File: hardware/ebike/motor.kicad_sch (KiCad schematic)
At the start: 48 parts, among them J2 Screw_Terminal_01x03, Q2 CSD19532KTT, Q3 CSD19532KTT, Q4 CSD19532KTT, Q5 CSD19532KTT, Q6 CSD19532KTT, Q7 CSD19532KTT

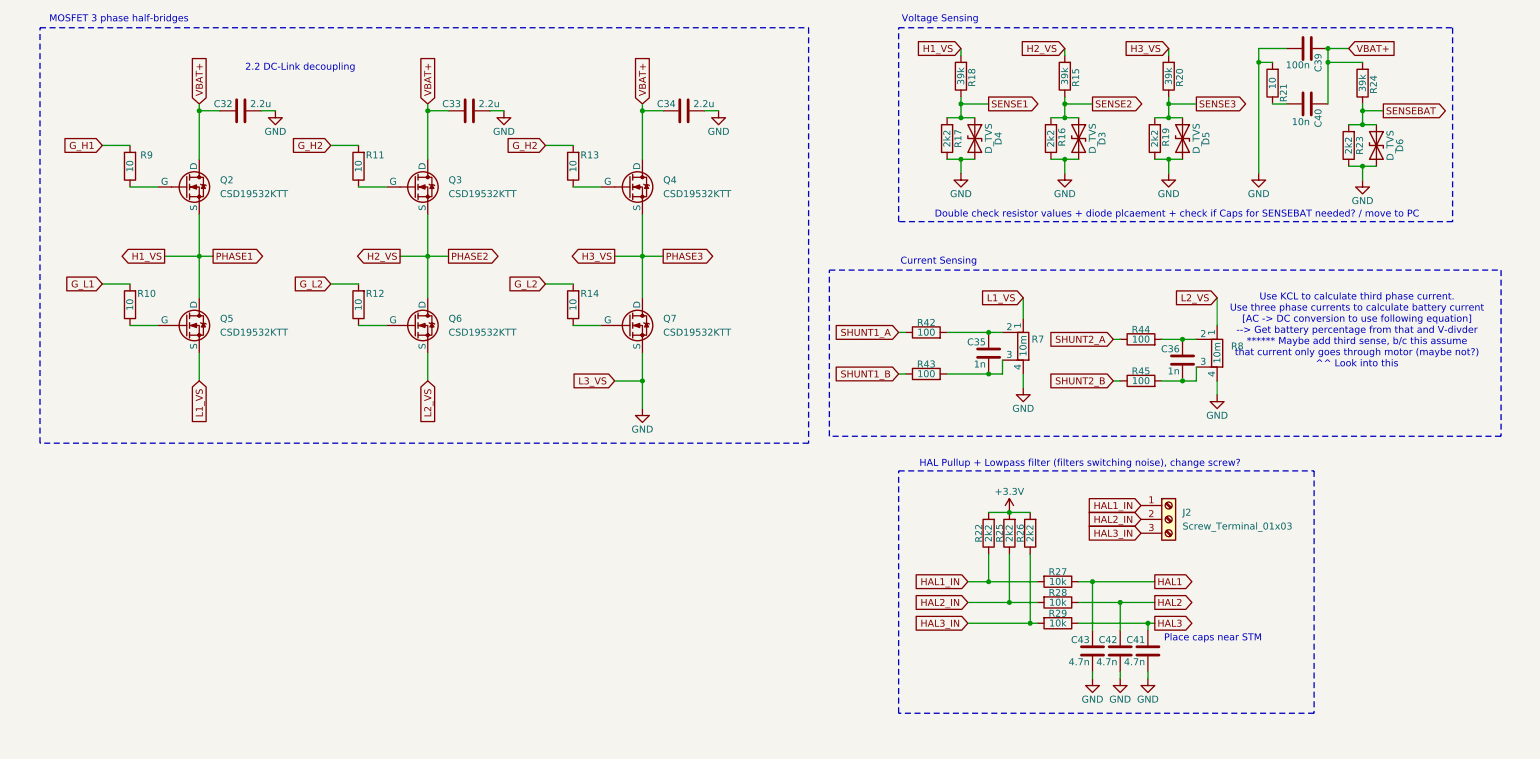
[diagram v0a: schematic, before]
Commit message: finished annoation for schematic
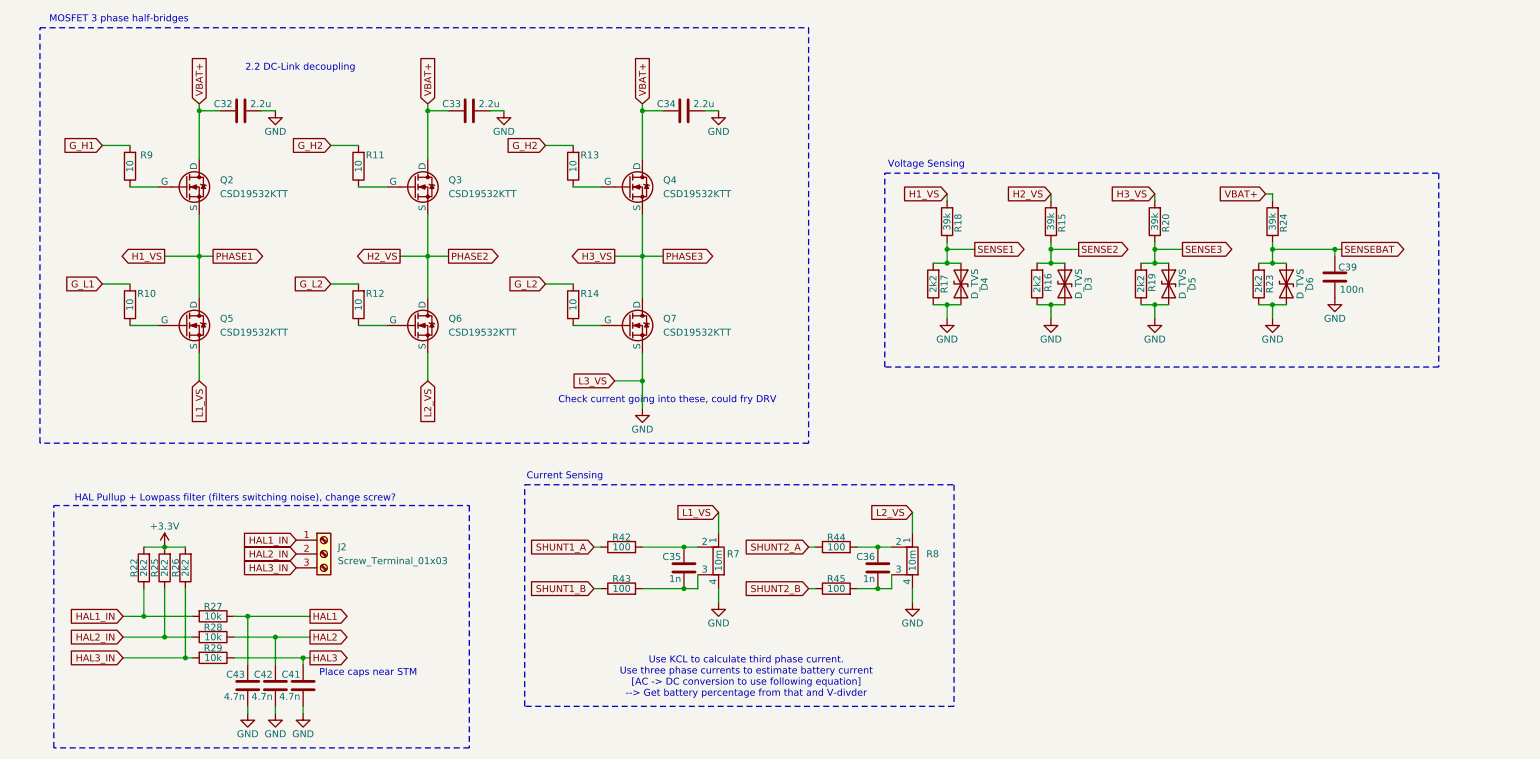
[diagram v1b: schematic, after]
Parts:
- removed C40: 10n, symbol Device:C
- removed R21: 10, symbol Device:R
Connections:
- net SENSEBAT: now also C39.2
- net VBAT+: no longer C39.2
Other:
- note added: "Check current going into these, could fry DRV"
- note added: "Use KCL to calculate third phase current. Use three phase currents to estimate battery current [AC -> DC conversion to use following equation] --> Get battery percentage from that and V-divder"
- note removed: "Double check resistor values + diode plcaement + check if Caps for SENSEBAT needed? / move to PC"
- note removed: "Use KCL to calculate third phase current. Use three phase currents to calculate battery current [AC -> DC conversion to use following equation] --> Get battery percentage from that and V-divder ****** Maybe add third sense, b/c this assume that current only goes through motor (maybe not?) ^^ Look into this"
- moved on the sheet: C35, C36, C39, C41, C42, C43, D3, D4, D5, D6, J2, R15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
